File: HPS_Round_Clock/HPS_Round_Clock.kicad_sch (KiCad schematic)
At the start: 144 parts, among them J1 Power_inlet_vertical, J2 Conn_01x06, SW1 Omron_B3F_SPST, SW2 Omron_B3F_SPST, SW3 Omron_B3F_SPST, SW4 Omron_B3F_SPST, SW5 Omron_B3F_SPST, U1 L7805, U2 DS1307_DIP-8, U4 ATmega328-PU, U5 TSOP38238, Y1 Crystal_16MHz, Y2 Crystal_32768Hz

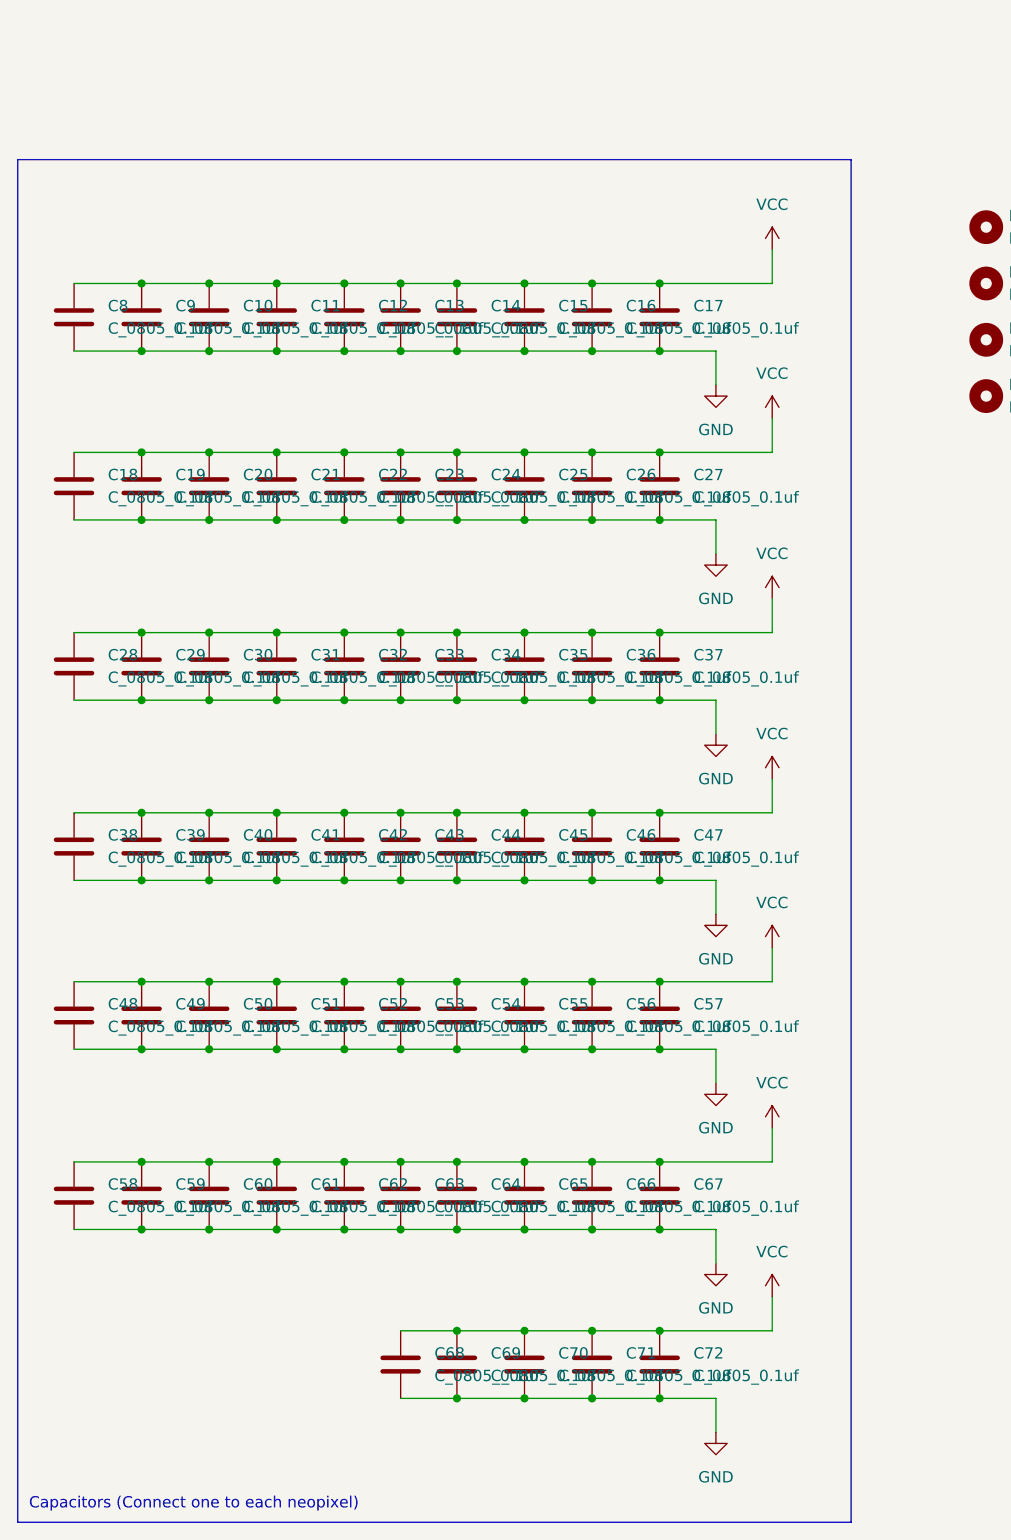
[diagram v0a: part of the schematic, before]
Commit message: Update HPS_Round_Clock.kicad_sch
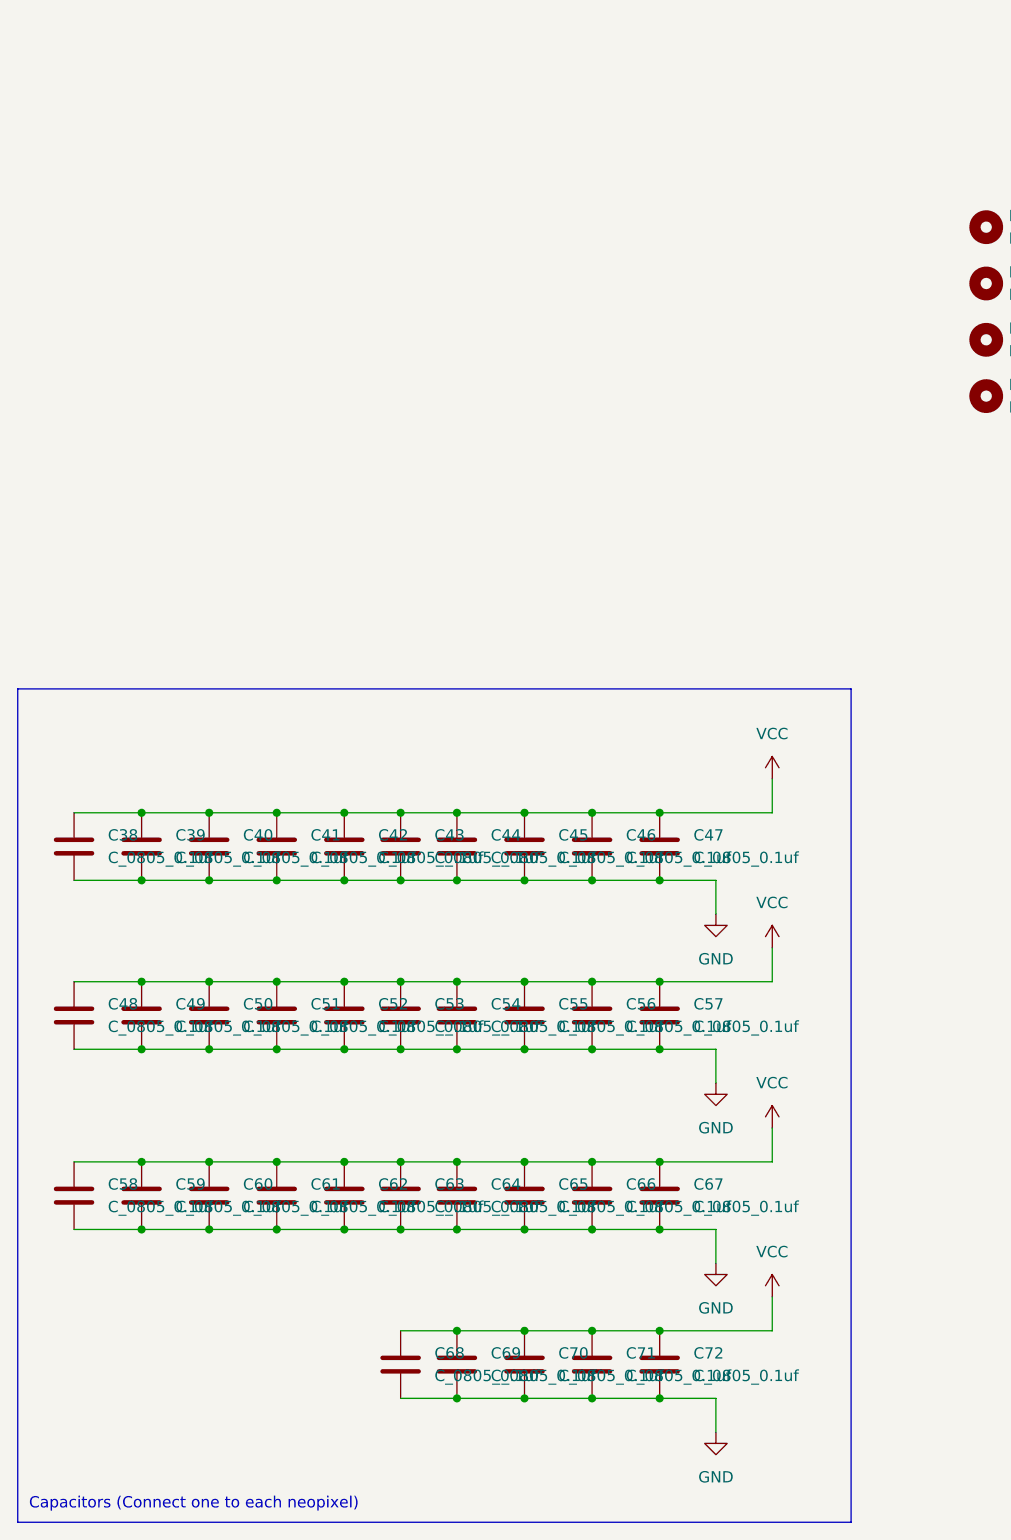
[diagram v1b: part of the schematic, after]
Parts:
- removed C10, C11, C12, C13, C14, C15, C16, C17, C18, C19, C20, C21, C22, C23, C24, C25, C26, C27, C28, C29, C30, C31, C32, C33, C34, C35, C36, C37, C8, C9: C_0805_0.1uf, footprints:C_0805_2012Metric, symbol HPS:C_0805_0.1uf
